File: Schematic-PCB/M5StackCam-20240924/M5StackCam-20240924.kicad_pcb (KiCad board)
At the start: 2 copper layers, 20.8 x 8.1 mm, 3 parts, among them J1 Conn_CamL, J2 Conn_CamR, J3 Conn_Main

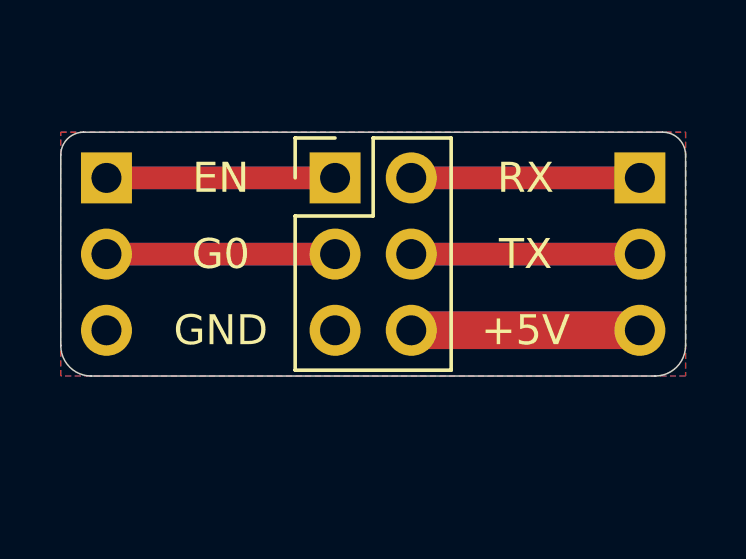
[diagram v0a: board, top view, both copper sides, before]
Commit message: update: カメラ用基板を更新した
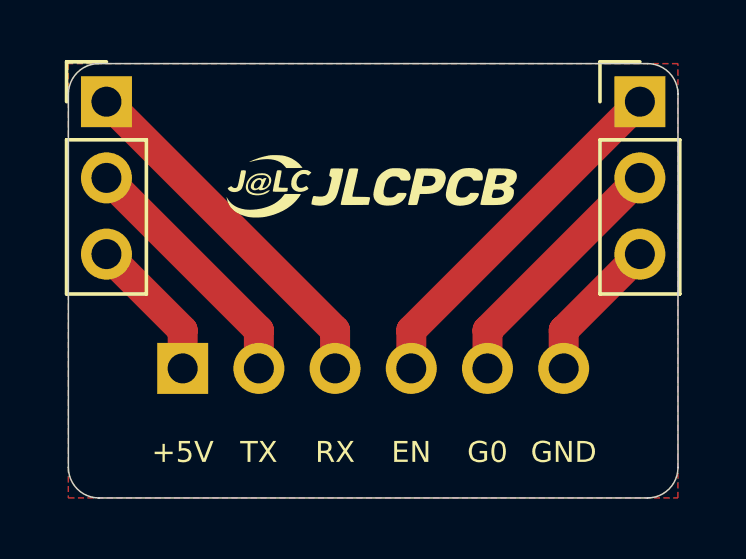
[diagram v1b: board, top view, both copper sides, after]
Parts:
- J1, J2: moved to F.Cu
- J3: value Conn_Main -> Conn_Output; footprint Connector_PinHeader_2.54mm:PinHeader_2x03_P2.54mm_Vertical -> Connector_PinHeader_2.54mm:PinHeader_1x06_P2.54mm_Horizontal; moved to B.Cu
- moved J1 18.0 mm to (17.8, -2.54), turned to 0 degrees
- moved J2 18.0 mm to (0.00, -2.54), turned to 0 degrees
- moved J3 8.13 mm to (2.54, 6.35), turned to -90 degrees
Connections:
- J3 pad 1: EN -> +5V
- J3 pad 2: RX -> TX
- J3 pad 3: G0 -> RX
- J3 pad 4: TX -> EN
- J3 pad 5: GND -> G0
- J3 pad 6: +5V -> GND
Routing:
- net +5V: track 15.2 -> 4.86 mm
- net TX: track 15.2 -> 8.45 mm
- net G0: track 15.2 -> 8.45 mm
- net GND: track 0.00 -> 4.86 mm
- net RX: track 15.2 -> 12.0 mm
- net EN: track 15.2 -> 12.0 mm
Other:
- board size 20.8 x 8.1 mm -> 20.3 x 14.5 mm
